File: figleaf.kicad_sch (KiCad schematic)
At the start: 5 parts, among them U1 Nice_Nano_V2

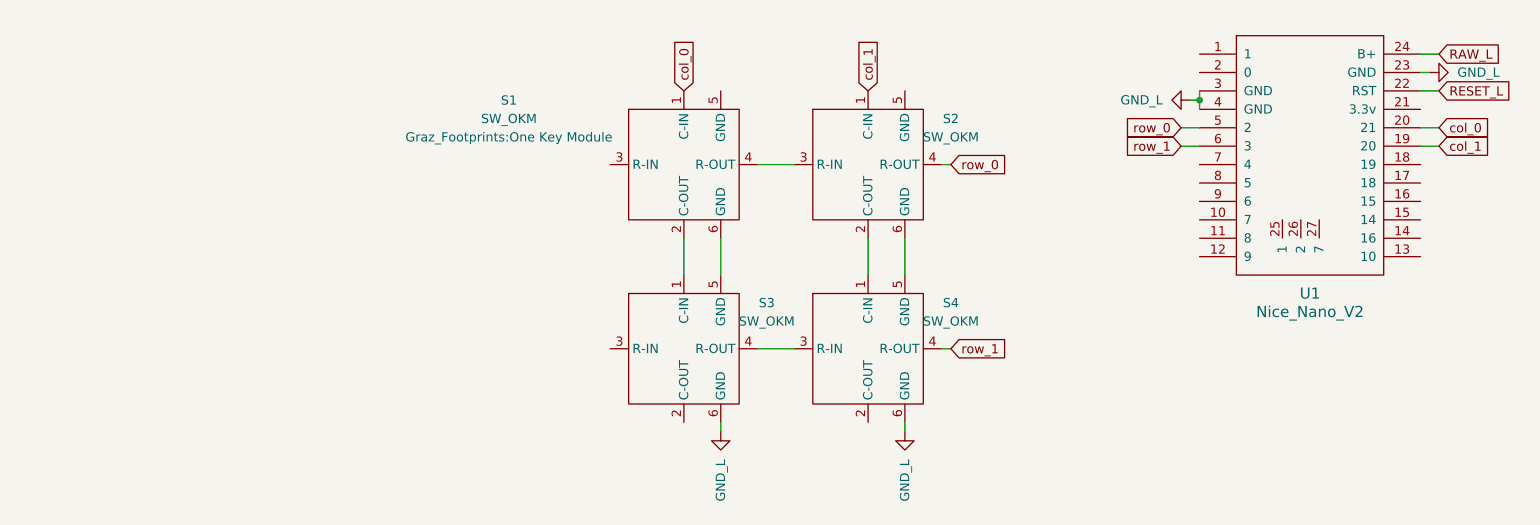
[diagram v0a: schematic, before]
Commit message: progress pcb
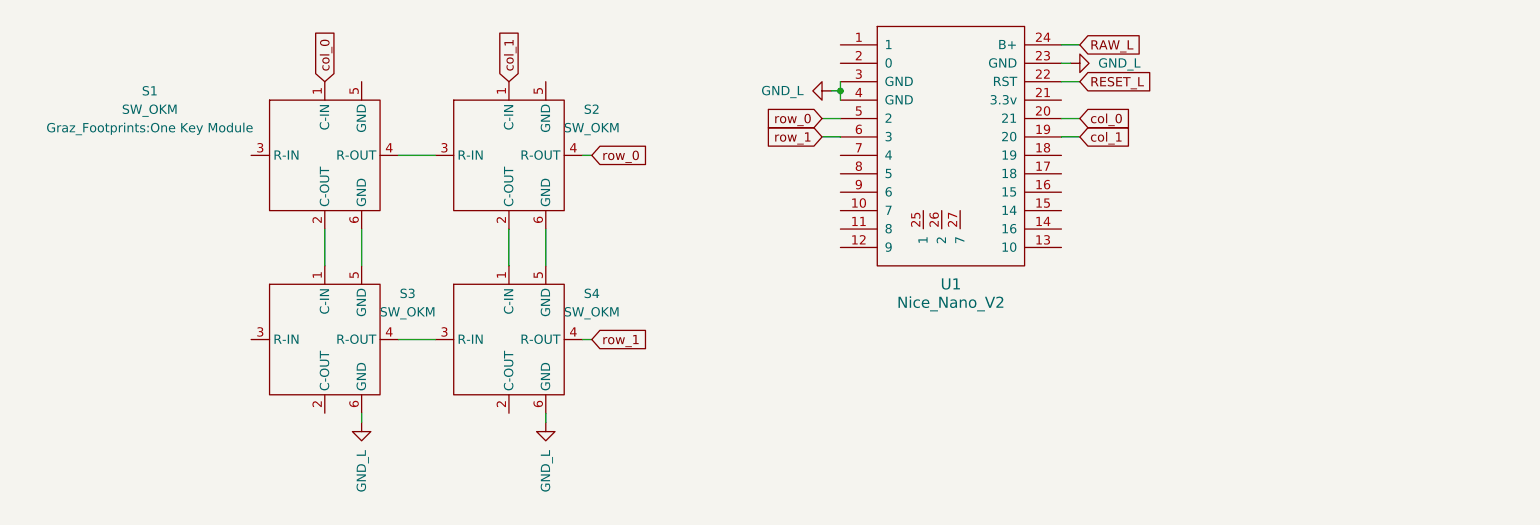
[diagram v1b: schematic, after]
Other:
- moved on the sheet: S1, S2, S3, S4, U1
